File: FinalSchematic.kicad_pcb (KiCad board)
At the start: 2 copper layers, 100 x 60.2 mm, 44 parts, among them IC1 SC-1020, J1 RF_Ant, J14 RX_Output, J6 TX_Input

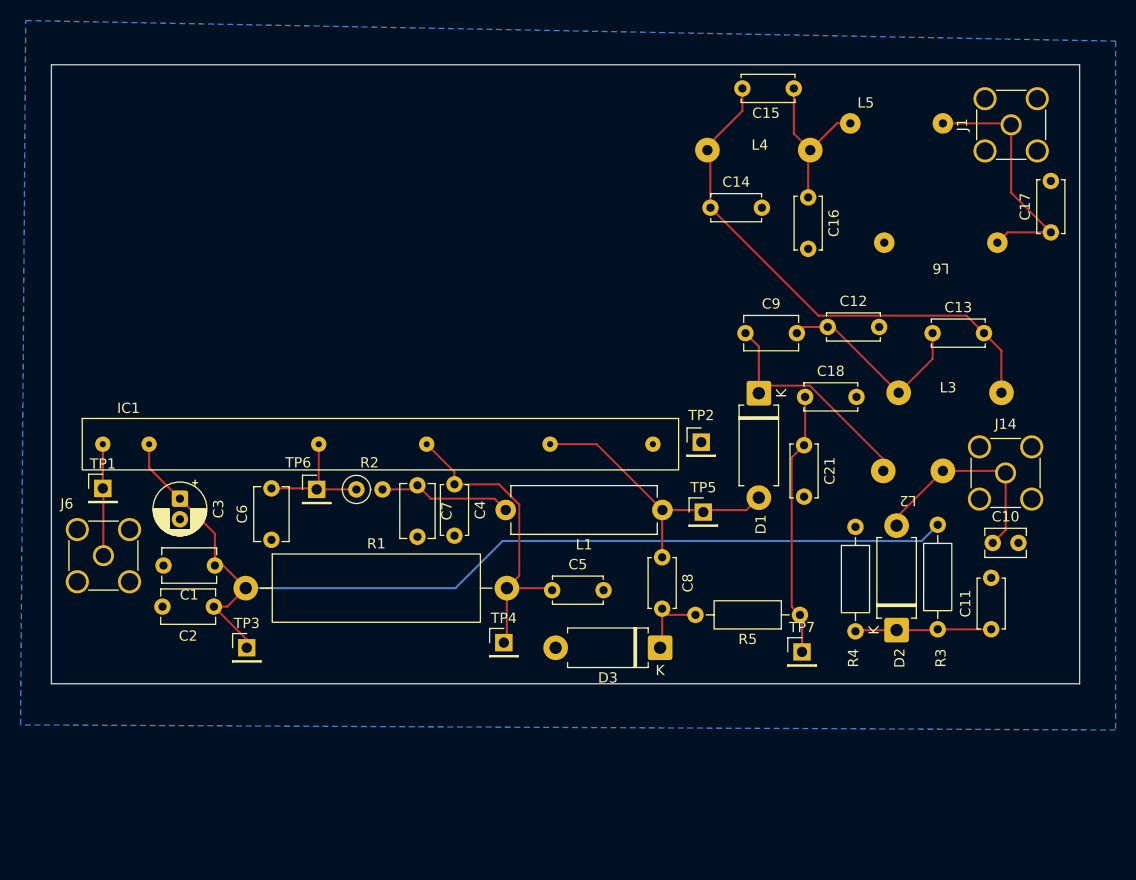
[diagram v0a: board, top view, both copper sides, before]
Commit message: Notes and Minor Tweaks
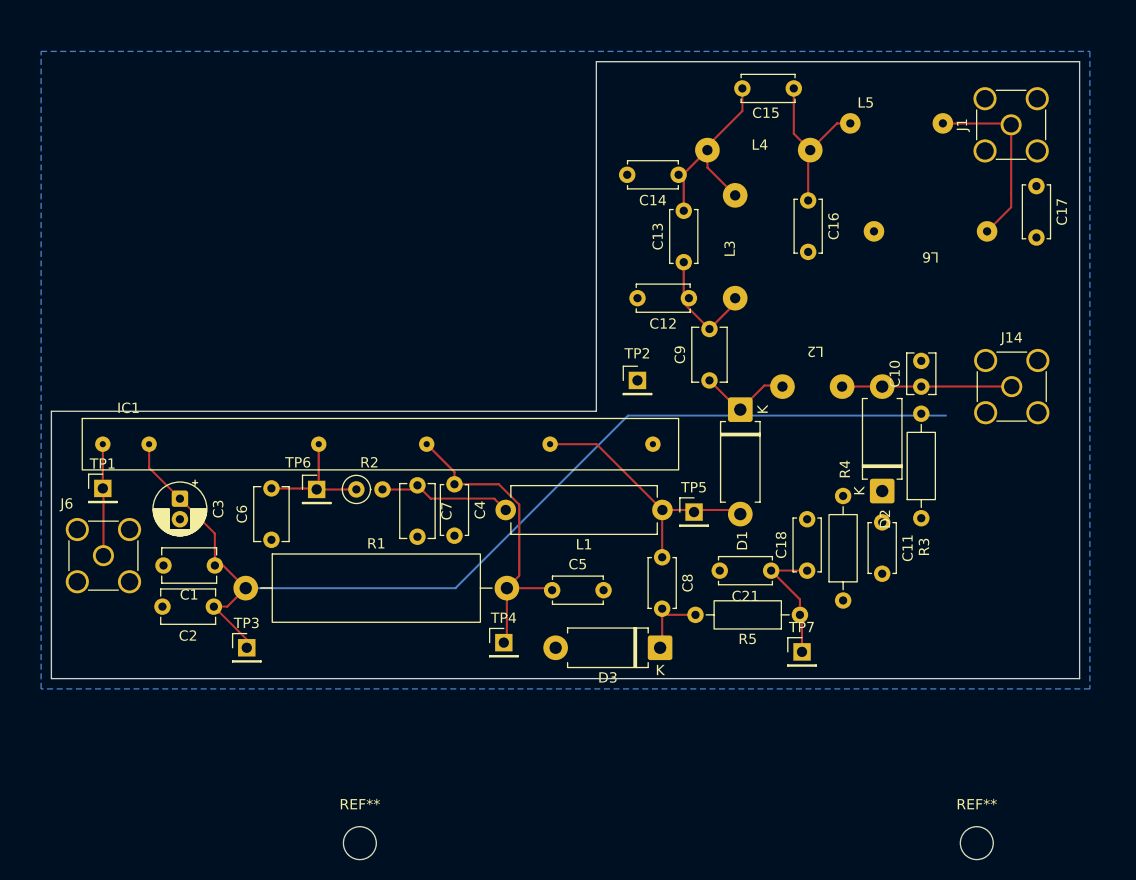
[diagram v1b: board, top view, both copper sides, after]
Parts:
- added REF**: MountingHole_3.2mm_M3_DIN965, MountingHole:MountingHole_3.2mm_M3_DIN965, F.Cu at (107.0, 112.0)
- added REF**: MountingHole_3.2mm_M3_DIN965, MountingHole:MountingHole_3.2mm_M3_DIN965, F.Cu at (167.0, 112.0)
- moved C13 25.2 mm to (138.5, 55.5), turned to 90 degrees
- moved L3 25.0 mm to (143.5, 54.2), turned to 90 degrees
- moved C18 16.9 mm to (150.5, 85.5), turned to 90 degrees
- moved C10 16.7 mm to (161.6, 67.6), turned to 90 degrees
- moved C11 14.8 mm to (157.8, 80.8), turned to -90 degrees
- moved C12 13.8 mm to (139.0, 59.0), turned to 180 degrees
- moved D2 13.6 mm to (157.8, 77.8)
- moved L2 12.8 mm to (153.9, 67.6)
- moved C21 12.6 mm to (147.0, 85.5), turned to 180 degrees
- moved R3 10.9 mm to (161.6, 80.4)
- moved TP2 8.63 mm to (134.0, 67.0)
- moved J14 8.42 mm to (170.4, 67.6)
- moved R4 7.26 mm to (154.0, 88.4), turned to 90 degrees
- moved C9 5.78 mm to (141.0, 67.0), turned to 90 degrees
- moved C17 4.71 mm to (172.8, 48.1), turned to -90 degrees
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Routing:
- net Net-(C13-Pad2): track 51.3 -> 20.9 mm
- net Net-(D1-K): track 22.9 -> 9.25 mm
- net Net-(D2-K): track 13.3 -> 0.00 mm
- net Net-(J2-Pin_1): track 25.8 -> 12.6 mm
- net Net-(C12-Pad1): track 20.0 -> 11.6 mm
- net Net-(J1-In): track 24.4 -> 18.0 mm
- net +12V: track 97.4 -> 102.6 mm
- net Net-(D2-A): track 20.7 -> 16.9 mm
- net Net-(D1-A): track 28.1 -> 26.4 mm
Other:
- board size 100 x 60.2 mm -> 100 x 60 mm
